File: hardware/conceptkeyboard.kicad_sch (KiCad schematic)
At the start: 73 parts, among them SW1 SW_Push, SW10 SW_Push, SW11 SW_Push, SW12 SW_Push, SW13 SW_Push, SW14 SW_Push, SW15 SW_Push, SW16 SW_Push, SW17 SW_Push, SW18 SW_Push, SW19 SW_Push, SW2 SW_Push, SW20 SW_Push, SW21 SW_Push, SW22 SW_Push, SW23 SW_Push, SW24 SW_Push, SW25 SW_Push, SW26 SW_Push, SW27 SW_Push, SW28 SW_Push, SW29 SW_Push, SW3 SW_Push, SW30 SW_Push, SW31 SW_Push, SW32 SW_Push, SW33 SW_Push, SW34 SW_Push, SW35 SW_Push, SW36 SW_Push, SW37 SW_Push, SW38 SW_Push, SW39 SW_Push, SW4 SW_Push, SW40 SW_Push, SW41 SW_Push, SW42 SW_Push, SW43 SW_Push, SW44 SW_Push, SW45 SW_Push, SW46 SW_Push, SW47 SW_Push, SW48 SW_Push, SW49 SW_Push, SW5 SW_Push, SW50 SW_Push, SW51 SW_Push, SW52 SW_Push, SW53 SW_Push, SW54 SW_Push, SW55 SW_Push, SW56 SW_Push, SW57 SW_Push, SW58 SW_Push, SW59 SW_Push, SW6 SW_Push, SW60 SW_Push, SW61 SW_Push, SW62 SW_Push, SW63 SW_Push, SW64 SW_Push, SW65 SW_Push, SW66 SW_Push, SW67 SW_Push, SW68 SW_Push, SW69 SW_Push, SW7 SW_Push, SW70 SW_Push, SW71 SW_Push, SW72 SW_Push, SW8 SW_Push, SW9 SW_Push, U1 STM32F103CBTx

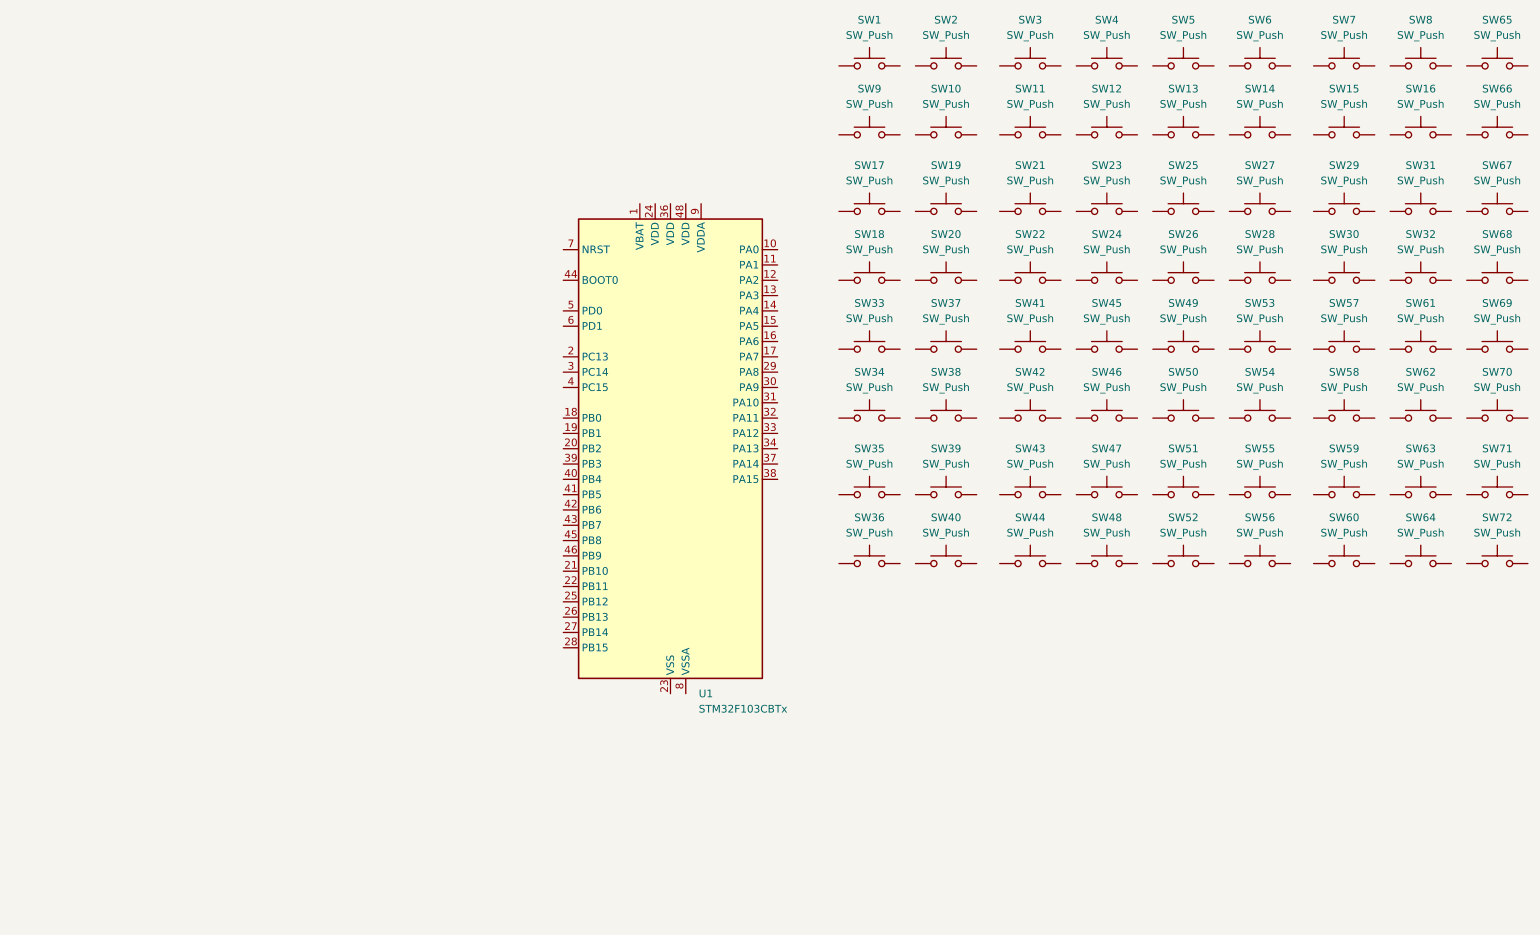
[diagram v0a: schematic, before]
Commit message: thingy
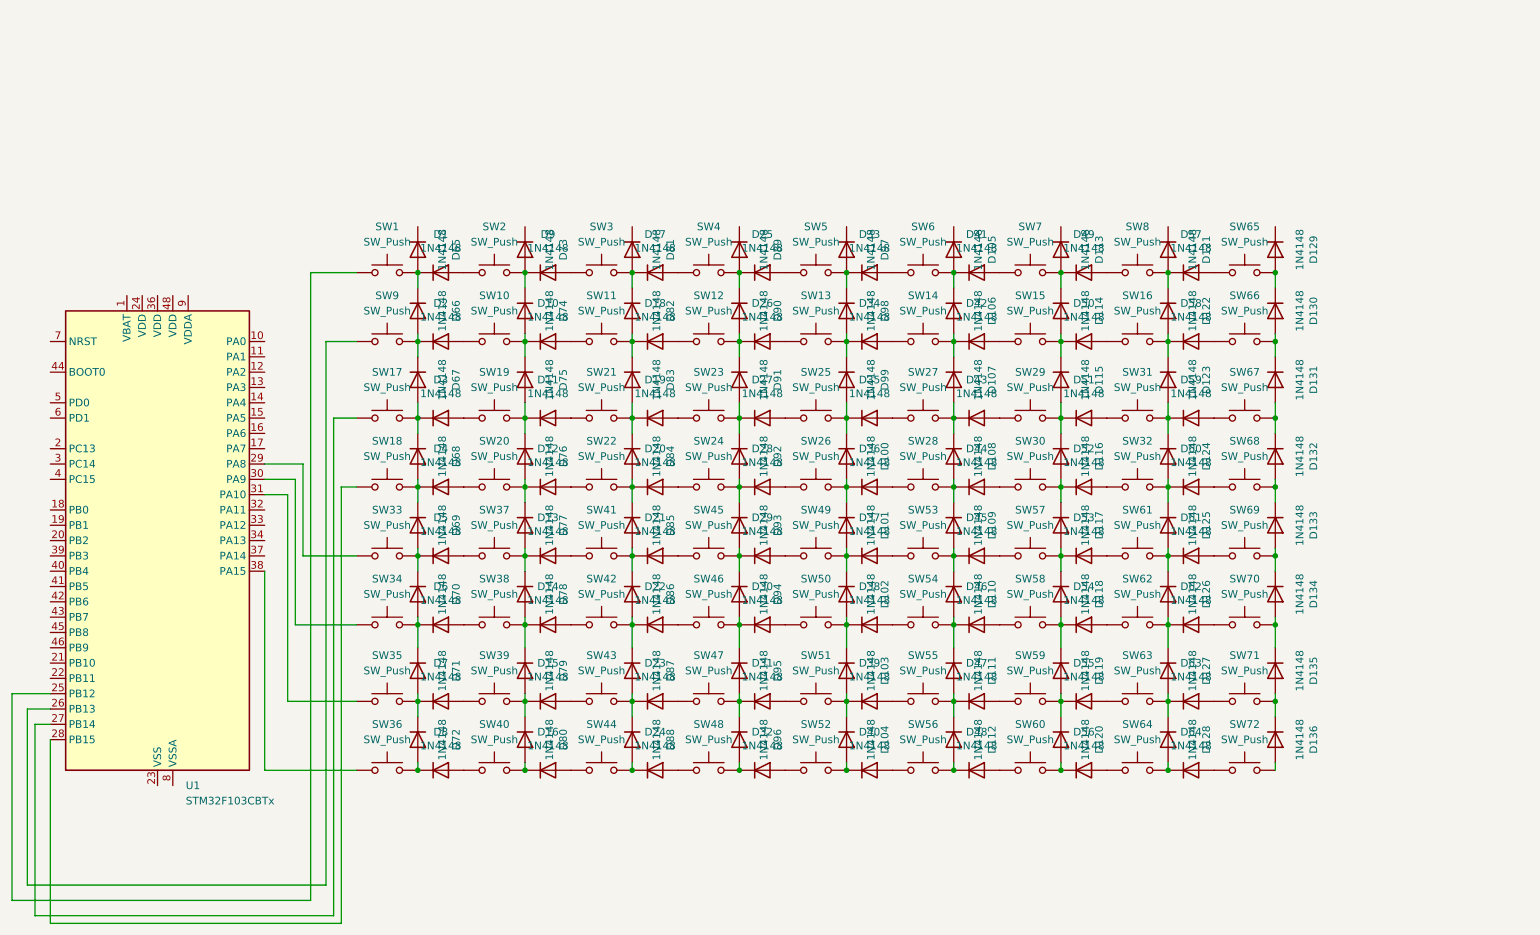
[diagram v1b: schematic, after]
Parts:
- added D1, D10, D100, D101, D102, D103, D104, D105, D106, D107, D108, D109, D11, D110, D111, D112, D113, D114, D115, D116, D117, D118, D119, D12, D120, D121, D122, D123, D124, D125, D126, D127, D128, D129, D13, D130, D131, D132, D133, D134, D135, D136, D14, D15, D16, D17, D18, D19, D2, D20, D21, D22, D23, D24, D25, D26, D27, D28, D29, D3, D30, D31, D32, D33, D34, D35, D36, D37, D38, D39, D4, D40, D41, D42, D43, D44, D45, D46, D47, D48, D49, D5, D50, D51, D52, D53, D54, D55, D56, D57, D58, D59, D6, D60, D61, D62, D63, D64, D65, D66, D67, D68, D69, D7, D70, D71, D72, D73, D74, D75, D76, D77, D78, D79, D8, D80, D81, D82, D83, D84, D85, D86, D87, D88, D89, D9, D90, D91, D92, D93, D94, D95, D96, D97, D98, D99: 1N4148, Diode_THT:D_DO-35_SOD27_P7.62mm_Horizontal, symbol Diode:1N4148
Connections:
- net at SW43.1: now also D15.2 (A)
- net at SW43.2: now also D23.1 (K), D87.2 (A), D88.1 (K)
- net at SW69.1: now also D61.2 (A)
- net at SW69.2: now also D133.2 (A), D134.1 (K)
- net at SW23.1: now also D19.2 (A)
- net at SW23.2: now also D27.1 (K), D91.2 (A), D92.1 (K)
- net at SW14.1: now also D34.2 (A)
- net at SW14.2: now also D106.2 (A), D107.1 (K), D42.1 (K)
- net at SW55.1: now also D39.2 (A)
- net at SW55.2: now also D111.2 (A), D112.1 (K), D47.1 (K)
- net at SW58.1: now also D46.2 (A)
- net at SW58.2: now also D118.2 (A), D119.1 (K), D54.1 (K)
- net at SW39.1: now also D7.2 (A)
- net at SW39.2: now also D15.1 (K), D79.2 (A), D80.1 (K)
- net at SW50.1: now also D30.2 (A)
- net at SW50.2: now also D102.2 (A), D103.1 (K), D38.1 (K)
- net at SW22.1: now also D12.2 (A)
- net at SW22.2: now also D20.1 (K), D84.2 (A), D85.1 (K)
- net at SW42.1: now also D14.2 (A)
- net at SW42.2: now also D22.1 (K), D86.2 (A), D87.1 (K)
- net at SW1.1: now also U1.25 (PB12)
- net at SW1.2: now also D1.1 (K), D65.2 (A), D66.1 (K)
- net at SW41.1: now also D13.2 (A)
- net at SW41.2: now also D21.1 (K), D85.2 (A), D86.1 (K)
- net at SW63.1: now also D55.2 (A)
- net at SW63.2: now also D127.2 (A), D128.1 (K), D63.1 (K)
- net at SW52.1: now also D32.2 (A)
- net at SW52.2: now also D104.2 (A), D40.1 (K)
- net at SW18.1: now also U1.28 (PB15)
- net at SW18.2: now also D4.1 (K), D68.2 (A), D69.1 (K)
- net at SW66.1: now also D58.2 (A)
- net at SW66.2: now also D130.2 (A), D131.1 (K)
- net at SW68.1: now also D60.2 (A)
- net at SW68.2: now also D132.2 (A), D133.1 (K)
- net at SW48.1: now also D24.2 (A)
- net at SW48.2: now also D32.1 (K), D96.2 (A)
- net at SW19.1: now also D3.2 (A)
- net at SW19.2: now also D11.1 (K), D75.2 (A), D76.1 (K)
- net at SW28.1: now also D36.2 (A)
- net at SW28.2: now also D108.2 (A), D109.1 (K), D44.1 (K)
- net at U1.26 (PB13): now also SW9.1
- net at U1.27 (PB14): now also SW17.1
- net at U1.29 (PA8): now also SW33.1
- net at U1.30 (PA9): now also SW34.1
- net at U1.31 (PA10): now also SW35.1
- net at U1.38 (PA15): now also SW36.1
- net at SW4.1: now also D17.2 (A)
- net at SW4.2: now also D25.1 (K), D89.2 (A), D90.1 (K)
- net at SW32.1: now also D52.2 (A)
- net at SW32.2: now also D124.2 (A), D125.1 (K), D60.1 (K)
- net at SW62.1: now also D54.2 (A)
- net at SW62.2: now also D126.2 (A), D127.1 (K), D62.1 (K)
- net at SW21.1: now also D11.2 (A)
- net at SW21.2: now also D19.1 (K), D83.2 (A), D84.1 (K)
- net at SW67.1: now also D59.2 (A)
- net at SW67.2: now also D131.2 (A), D132.1 (K)
- net at SW71.1: now also D63.2 (A)
- net at SW71.2: now also D135.2 (A), D136.1 (K)
- net at SW26.1: now also D28.2 (A)
- net at SW26.2: now also D100.2 (A), D101.1 (K), D36.1 (K)
- net at SW10.1: now also D2.2 (A)
- net at SW10.2: now also D10.1 (K), D74.2 (A), D75.1 (K)
- net at SW70.1: now also D62.2 (A)
- net at SW70.2: now also D134.2 (A), D135.1 (K)
- net at SW51.1: now also D31.2 (A)
- net at SW51.2: now also D103.2 (A), D104.1 (K), D39.1 (K)
- net at SW65.1: now also D57.2 (A)
- net at SW65.2: now also D129.2 (A), D130.1 (K)
- net at SW37.1: now also D5.2 (A)
- net at SW37.2: now also D13.1 (K), D77.2 (A), D78.1 (K)
- net at SW36.2: now also D72.2 (A), D8.1 (K)
- net at SW17.2: now also D3.1 (K), D67.2 (A), D68.1 (K)
- net at SW61.1: now also D53.2 (A)
- net at SW61.2: now also D125.2 (A), D126.1 (K), D61.1 (K)
- net at SW45.1: now also D21.2 (A)
- net at SW45.2: now also D29.1 (K), D93.2 (A), D94.1 (K)
- net at SW30.1: now also D44.2 (A)
- net at SW30.2: now also D116.2 (A), D117.1 (K), D52.1 (K)
- net at SW54.1: now also D38.2 (A)
- net at SW54.2: now also D110.2 (A), D111.1 (K), D46.1 (K)
- net at SW6.1: now also D33.2 (A)
- net at SW6.2: now also D105.2 (A), D106.1 (K), D41.1 (K)
- net at SW47.1: now also D23.2 (A)
- net at SW47.2: now also D31.1 (K), D95.2 (A), D96.1 (K)
- net at SW7.1: now also D41.2 (A)
- net at SW7.2: now also D113.2 (A), D114.1 (K), D49.1 (K)
- net at SW38.1: now also D6.2 (A)
- net at SW38.2: now also D14.1 (K), D78.2 (A), D79.1 (K)
- net at SW35.2: now also D7.1 (K), D71.2 (A), D72.1 (K)
- net at SW9.2: now also D2.1 (K), D66.2 (A), D67.1 (K)
- net at SW59.1: now also D47.2 (A)
- net at SW59.2: now also D119.2 (A), D120.1 (K), D55.1 (K)
- net at SW29.1: now also D43.2 (A)
- net at SW29.2: now also D115.2 (A), D116.1 (K), D51.1 (K)
- net at SW5.1: now also D25.2 (A)
- net at SW5.2: now also D33.1 (K), D97.2 (A), D98.1 (K)
- net at SW8.1: now also D49.2 (A)
- net at SW8.2: now also D121.2 (A), D122.1 (K), D57.1 (K)
- net at SW34.2: now also D6.1 (K), D70.2 (A), D71.1 (K)
- net at SW20.1: now also D4.2 (A)
- net at SW20.2: now also D12.1 (K), D76.2 (A), D77.1 (K)
- net at SW40.1: now also D8.2 (A)
- net at SW40.2: now also D16.1 (K), D80.2 (A)
- net at SW44.1: now also D16.2 (A)
- net at SW44.2: now also D24.1 (K), D88.2 (A)
- net at SW27.1: now also D35.2 (A)
- net at SW27.2: now also D107.2 (A), D108.1 (K), D43.1 (K)
- net at SW49.1: now also D29.2 (A)
- net at SW49.2: now also D101.2 (A), D102.1 (K), D37.1 (K)
- net at SW25.1: now also D27.2 (A)
- net at SW25.2: now also D100.1 (K), D35.1 (K), D99.2 (A)
- net at SW72.1: now also D64.2 (A)
- net at SW72.2: now also D136.2 (A)
- net at SW46.1: now also D22.2 (A)
- net at SW46.2: now also D30.1 (K), D94.2 (A), D95.1 (K)
- net at SW31.1: now also D51.2 (A)
- net at SW31.2: now also D123.2 (A), D124.1 (K), D59.1 (K)
- net at SW3.1: now also D9.2 (A)
- net at SW3.2: now also D17.1 (K), D81.2 (A), D82.1 (K)
- net at SW16.1: now also D50.2 (A)
- net at SW16.2: now also D122.2 (A), D123.1 (K), D58.1 (K)
- net at SW15.1: now also D42.2 (A)
- net at SW15.2: now also D114.2 (A), D115.1 (K), D50.1 (K)
- net at SW13.1: now also D26.2 (A)
- net at SW13.2: now also D34.1 (K), D98.2 (A), D99.1 (K)
- net at SW24.1: now also D20.2 (A)
- net at SW24.2: now also D28.1 (K), D92.2 (A), D93.1 (K)
- net at SW2.1: now also D1.2 (A)
- net at SW2.2: now also D73.2 (A), D74.1 (K), D9.1 (K)
- net at SW56.1: now also D40.2 (A)
- net at SW56.2: now also D112.2 (A), D48.1 (K)
- net at SW11.1: now also D10.2 (A)
- net at SW11.2: now also D18.1 (K), D82.2 (A), D83.1 (K)
- net at SW60.1: now also D48.2 (A)
- net at SW60.2: now also D120.2 (A), D56.1 (K)
- net at SW57.1: now also D45.2 (A)
- net at SW57.2: now also D117.2 (A), D118.1 (K), D53.1 (K)
- net at SW64.1: now also D56.2 (A)
- net at SW64.2: now also D128.2 (A), D64.1 (K)
- net at SW12.1: now also D18.2 (A)
- net at SW12.2: now also D26.1 (K), D90.2 (A), D91.1 (K)
- net at SW33.2: now also D5.1 (K), D69.2 (A), D70.1 (K)
- net at SW53.1: now also D37.2 (A)
- net at SW53.2: now also D109.2 (A), D110.1 (K), D45.1 (K)
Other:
- moved on the sheet: SW1, SW10, SW11, SW12, SW13, SW14, SW15, SW16, SW17, SW18, SW19, SW2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
